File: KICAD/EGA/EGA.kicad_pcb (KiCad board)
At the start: 2 copper layers, 162.2 x 134 mm, 39 parts, among them J1 12V, J10 TEST_TRIG, J2 HC-SR04, J3 LCD 20x4, J4 RTC, J5 TEST_PWM, J6 FAN_12V_PWM_3.3V, J7 UART, J8 TEST_RPM, J9 TEST_ECHO, SW1 PAGINA, SW2 RESET, U1 LM7805_TO220, U2 LM317_TO-220, U3 Pico

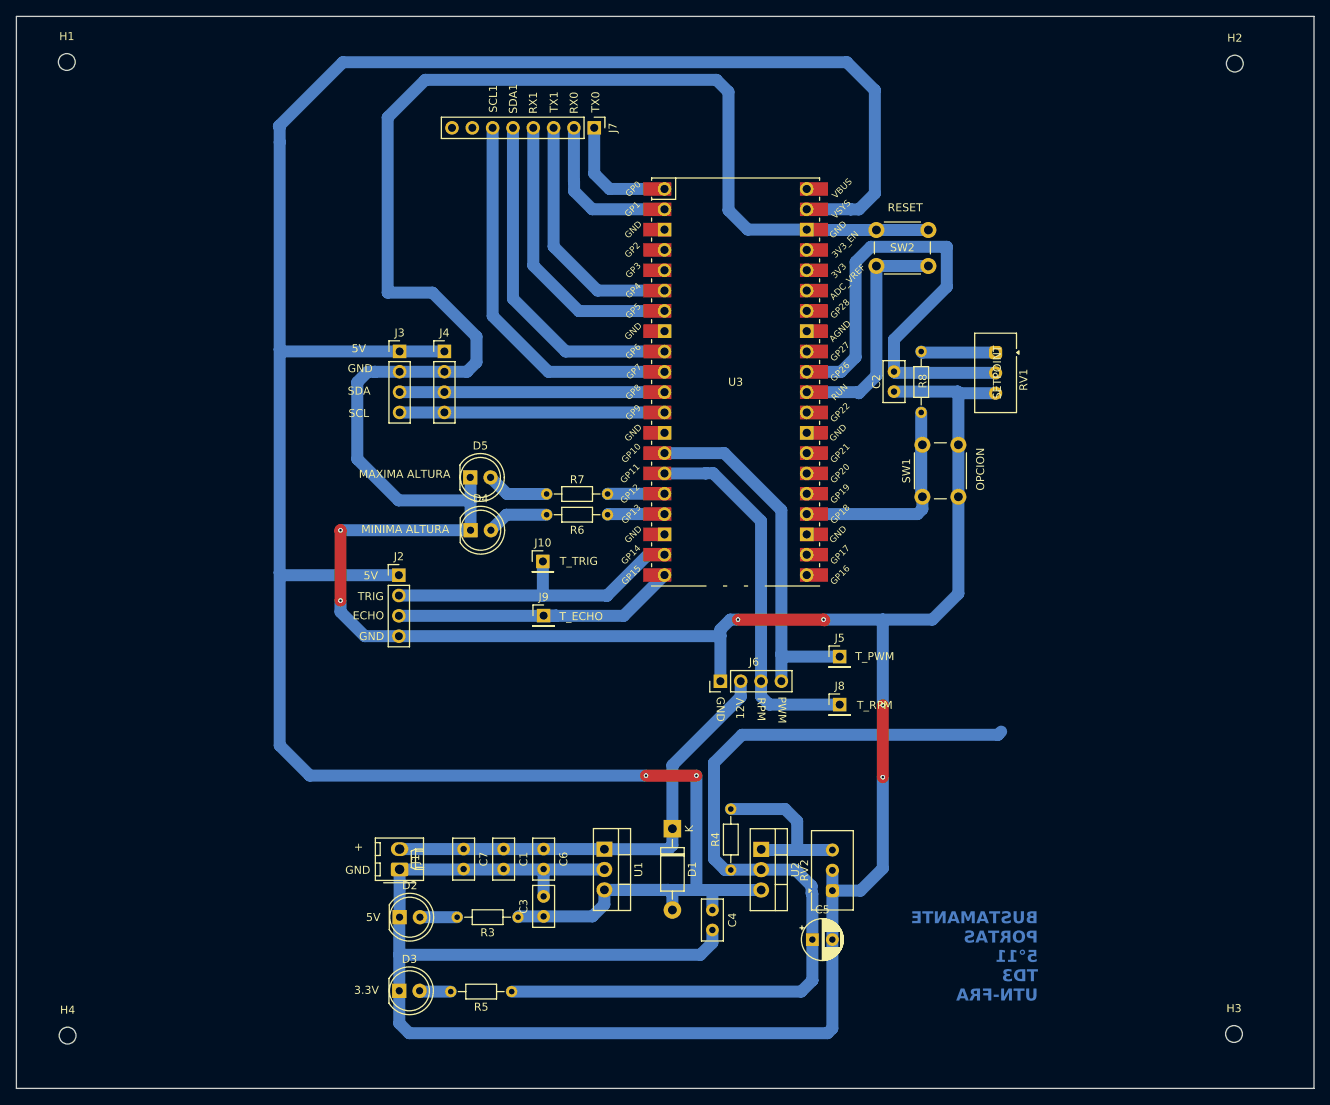
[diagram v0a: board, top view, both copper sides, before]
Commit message: features/Rama Agregado de SD
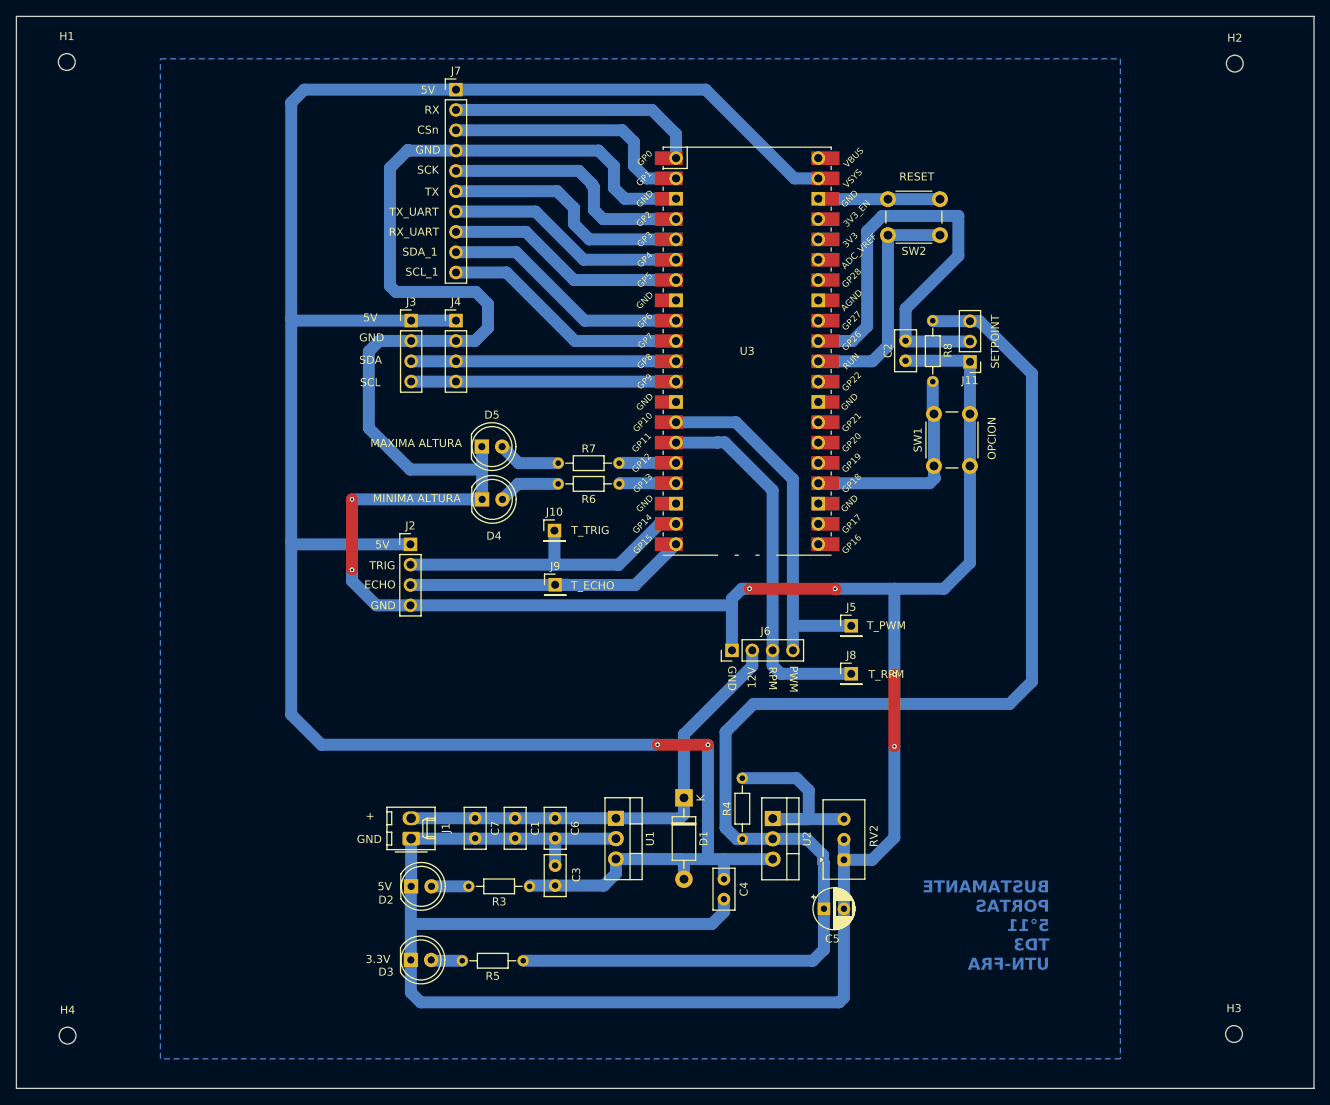
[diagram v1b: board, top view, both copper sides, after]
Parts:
- removed RV1: SetPoint, Potentiometer_THT:Potentiometer_Vishay_T93XA_Horizontal
- added J11: POTENCIOMETRO, Connector_PinHeader_2.54mm:PinHeader_1x03_P2.54mm_Vertical, F.Cu at (156.2, 67.9)
- J7: footprint Connector_PinHeader_2.54mm:PinHeader_1x08_P2.54mm_Vertical -> Connector_PinHeader_2.54mm:PinHeader_1x10_P2.54mm_Vertical
- SW1, SW2: footprint Button_Switch_THT:SW_PUSH_6mm_H5mm -> Button_Switch_THT:SW_PUSH_6mm_H8mm
- moved J7 17.9 mm to (91.9, 33.9), turned to 0 degrees
- moved R3 4.12 mm to (101.2, 133.4)
- moved C4 4.12 mm to (125.4, 132.5)
- moved D2 4.12 mm to (86.3, 133.4)
- moved U1 4.12 mm to (111.9, 124.9)
- moved D4 4.12 mm to (95.2, 85.1)
- moved R4 4.12 mm to (127.7, 127.5)
- moved D5 4.12 mm to (95.2, 78.5)
- moved J10 4.12 mm to (104.3, 89.0)
- moved J2 4.12 mm to (86.3, 90.7)
- moved J5 4.12 mm to (141.4, 100.9)
- moved J6 4.12 mm to (126.4, 103.9)
- moved J8 4.12 mm to (141.4, 106.9)
- moved R7 4.12 mm to (112.3, 80.5)
- moved R8 4.12 mm to (151.5, 62.7)
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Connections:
- J7 pad 1: UART0_TX -> 5V
- J7 pad 2: UART0_RX -> RX/SPI0
- J7 pad 3: UART1_TX -> CSn/SPI0
- J7 pad 4: UART1_RX -> GND
- J7 pad 5: SDA_1 -> SCK/SPI0
- J7 pad 6: SCL_1 -> TX/SPI0
- J7 pad 7: unconnected-(J7-Pin_7-Pad7) -> UART1_TX
- J7 pad 8: unconnected-(J7-Pin_8-Pad8) -> UART1_RX
- SW2 pad 2: GND -> Net-(SW2-Pad2)
- U3 pad 1: UART0_TX -> RX/SPI0
- U3 pad 2: UART0_RX -> CSn/SPI0
- U3 pad 3: unconnected-(U3-GND-Pad3) -> GND
- U3 pad 38: GND -> Net-(SW2-Pad2)
- U3 pad 4: unconnected-(U3-GPIO2-Pad4)_0 -> SCK/SPI0
- U3 pad 5: unconnected-(U3-GPIO3-Pad5) -> TX/SPI0
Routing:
- net GND: track 527.5 -> 470.0 mm
- net 3.3V: track 122.5 -> 170.2 mm
- net RX/SPI0: track 0.00 -> 31.8 mm
- net SCK/SPI0: track 0.00 -> 31.8 mm
- net CSn/SPI0: track 0.00 -> 31.8 mm
- net 5V: track 328.9 -> 297.5 mm
- net TX/SPI0: track 0.00 -> 31.2 mm
- net UART0_RX: track 20.2 -> 0.00 mm
- net SCL_1: track 47.9 -> 31.1 mm
- net Net-(SW2-Pad2): track 0.00 -> 15.3 mm
- net UART0_TX: track 15.3 -> 0.00 mm
- net SDA_1: track 43.0 -> 31.1 mm
- net UART1_RX: track 36.0 -> 30.2 mm
- net PIN_ADC: track 62.1 -> 57.4 mm
- net UART1_TX: track 31.0 -> 30.0 mm
- added copper zone on B.Cu, net GND
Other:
- board text added: "CSn"
- board text added: "RX"
- board text added: "RX_UART"
- board text added: "SCK"
- board text added: "SCL_1"
- board text added: "SDA_1"
- board text added: "TX"
- board text added: "TX_UART"
- board text removed: "RX0"
- board text removed: "RX1"
- board text removed: "SCL1"
- board text removed: "SDA1"
- board text removed: "TX0"
- board text removed: "TX1"
